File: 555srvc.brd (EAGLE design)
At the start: 20.5 x 7.9 mm, 10 parts, among them IC1 555

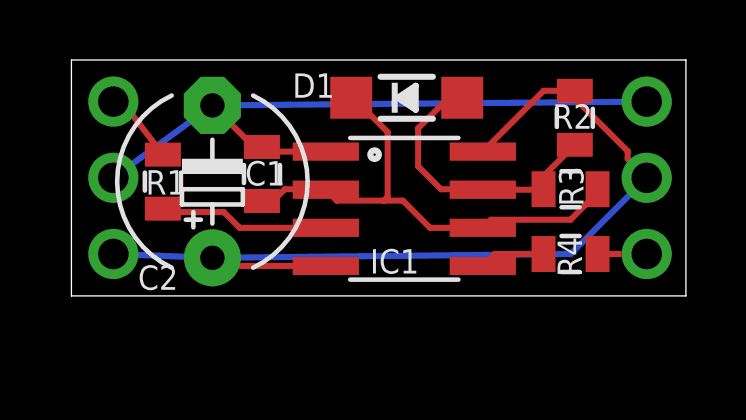
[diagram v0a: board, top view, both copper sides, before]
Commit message: looks legit
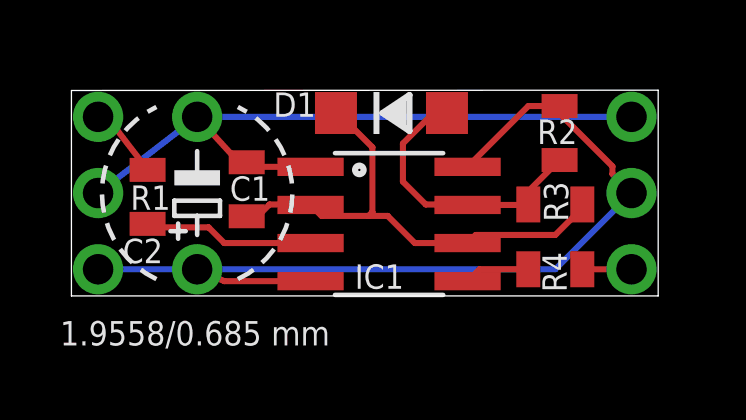
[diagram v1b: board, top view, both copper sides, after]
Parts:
- moved R2 0.72 mm to (16.3, 5.43)
- moved D1 0.72 mm to (10.7, 6.10)
- moved IC1 0.72 mm to (10.6, 2.40)
- moved C1 0.72 mm to (5.84, 3.56)
- moved JP2 0.72 mm to (0.89, 3.43)
- moved R1 0.72 mm to (2.54, 3.30)
- moved JP3 0.72 mm to (18.7, 3.43)
- moved R3 0.72 mm to (16.1, 3.05)
- moved R4 0.72 mm to (16.1, 0.89)
- moved C2 0.64 mm to (4.19, 3.43)
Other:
- board size 20.5 x 7.9 mm -> 19.6 x 6.9 mm
- board text added: "1.9558/0.685 mm"
